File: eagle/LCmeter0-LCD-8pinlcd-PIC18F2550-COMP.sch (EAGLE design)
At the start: 35 parts, among them IC1 PIC18F2550-I/SP-COMP-B-V, J1 HD44780-4BITLCD44780-8P, J2 PIC-UART, J3 PIC-ICSP, J4 J4, J5 CONN-2P2P/V, J7 CONN-2P2P/V, K2 DS2Y, Q1 20MHz, SW1 PB-1P-1T, T1 BC547

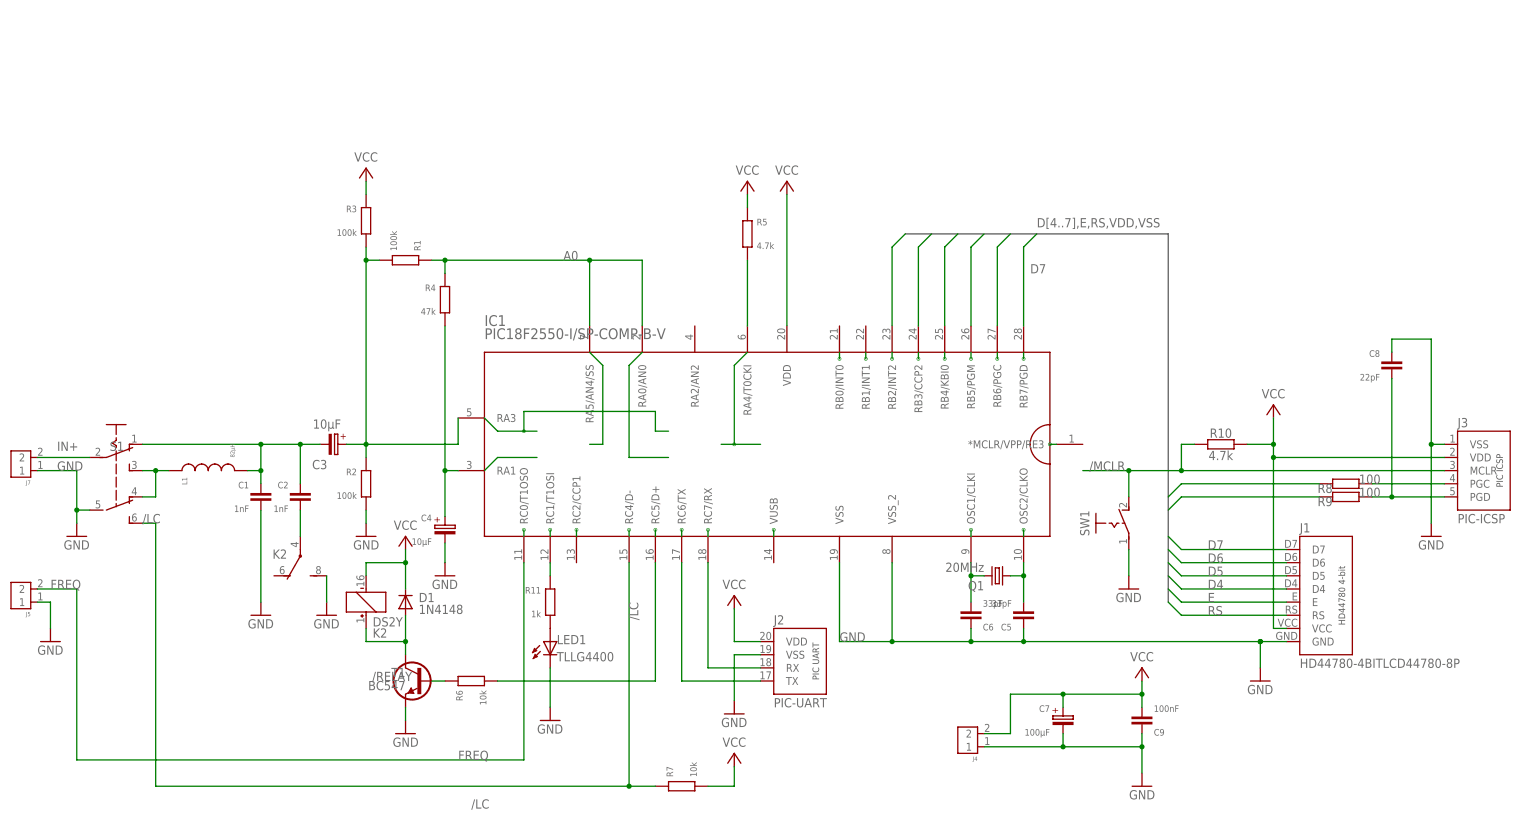
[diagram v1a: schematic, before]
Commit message: ...
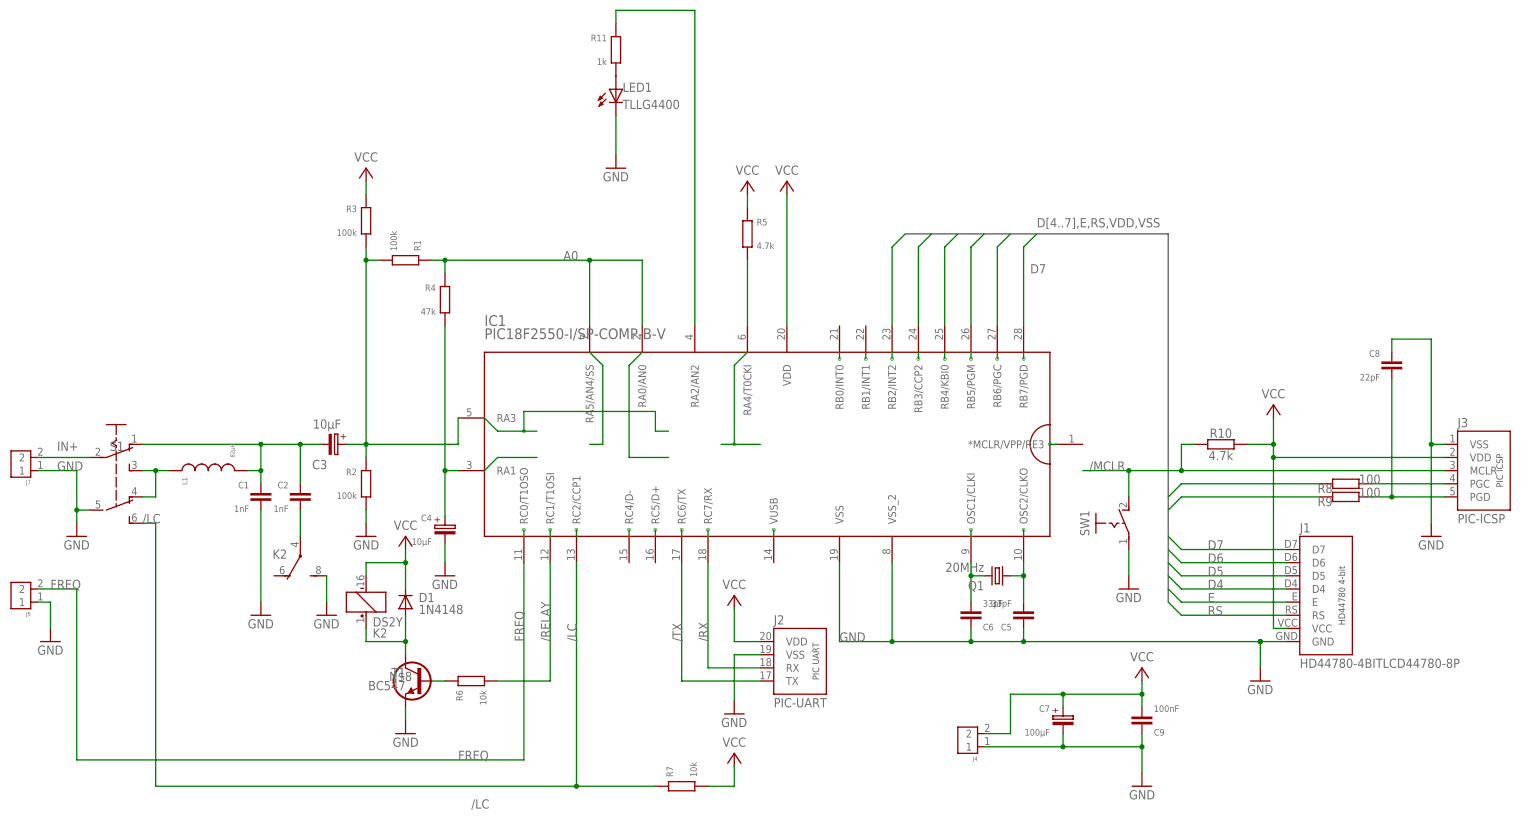
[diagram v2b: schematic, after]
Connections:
- net N$10 renamed /TX
- net N$9 renamed /RX
- net /LC: now also IC1.RC2/CCP1; no longer IC1.RC4/D-
- net /RELAY: now also IC1.RC1/T1OSI, R6.1; no longer D1.A, K21.+, T1.C
- net N$3: now also IC1.RA2/AN2; no longer IC1.RC1/T1OSI
- net N$8: now also D1.A, K21.+, T1.C; no longer IC1.RC5/D+, R6.1
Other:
- moved on the sheet: LED1, R11
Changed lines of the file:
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@@
 </instance>
 <instance part="J1" gate="G$1" x="228.6" y="0"/>
-<instance part="LED1" gate="G$1" x="86.36" y="-8.89" rot="MR0"/>
-<instance part="GND10" gate="1" x="86.36" y="-22.86"/>
+<instance part="LED1" gate="G$1" x="99.06" y="97.79" rot="MR0"/>
+<instance part="GND10" gate="1" x="99.06" y="83.82"/>
 <instance part="GND13" gate="1" x="200.66" y="-35.56" rot="MR0"/>
 <instance part="J4" gate="G$1" x="167.64" y="-27.94" rot="MR0"/>
@@
 </instance>
 <instance part="R6" gate="G$1" x="71.12" y="-15.24" rot="R90"/>
-<instance part="R11" gate="G$1" x="86.36" y="0"/>
+<instance part="R11" gate="G$1" x="99.06" y="106.68"/>
 <instance part="J7" gate="G$1" x="-15.24" y="25.4" rot="MR0"/>
 <instance part="J5" gate="G$1" x="-15.24" y="0" rot="MR0"/>
@@
 <pinref part="GND10" gate="1" pin="GND"/>
 <pinref part="LED1" gate="G$1" pin="C"/>
-<wire x1="86.36" y1="-12.7" x2="86.36" y2="-20.32" width="0.1524" layer="91"/>
+<wire x1="99.06" y1="93.98" x2="99.06" y2="86.36" width="0.1524" layer="91"/>
 </segment>
 <segment>
@@
 <pinref part="S1" gate="G$1" pin="S1"/>
 <wire x1="10.16" y1="15.24" x2="10.16" y2="-35.56" width="0.1524" layer="91"/>
-<wire x1="10.16" y1="-35.56" x2="101.6" y2="-35.56" width="0.1524" layer="91"/>
+<wire x1="10.16" y1="-35.56" x2="91.44" y2="-35.56" width="0.1524" layer="91"/>
 <label x="71.12" y="-38.1" size="1.778" layer="95" rot="MR180"/>
 <pinref part="R7" gate="G$1" pin="2"/>
-<wire x1="101.6" y1="7.62" x2="101.6" y2="-35.56" width="0.1524" layer="91"/>
-<wire x1="101.6" y1="-35.56" x2="106.68" y2="-35.56" width="0.1524" layer="91"/>
-<junction x="101.6" y="-35.56"/>
-<label x="101.6" y="0" size="1.778" layer="95" rot="R270"/>
-<pinref part="IC1" gate="G$1" pin="RC4/D-"/>
-</segment>
-</net>
-<net name="/RELAY" class="0">
+<pinref part="IC1" gate="G$1" pin="RC2/CCP1"/>
+<wire x1="91.44" y1="-35.56" x2="106.68" y2="-35.56" width="0.1524" layer="91"/>
+<wire x1="91.44" y1="-35.56" x2="91.44" y2="7.62" width="0.1524" layer="91"/>
+<junction x="91.44" y="-35.56"/>
+<label x="91.44" y="-7.62" size="1.778" layer="95" rot="R90"/>
+</segment>
+</net>
+<net name="N$8" class="0">
 <segment>
 <pinref part="T1" gate="G$1" pin="C"/>
@@
 <label x="68.58" y="-30.48" size="1.778" layer="95"/>
 <pinref part="IC1" gate="G$1" pin="RC0/T1OSO"/>
+<label x="81.28" y="-7.62" size="1.778" layer="95" rot="R90"/>
 </segment>
 </net>
@@
 </segment>
 </net>
-<net name="N$8" class="0">
+<net name="/RELAY" class="0">
 <segment>
 <pinref part="R6" gate="G$1" pin="1"/>
-<wire x1="76.2" y1="-15.24" x2="106.68" y2="-15.24" width="0.1524" layer="91"/>
-<wire x1="106.68" y1="-15.24" x2="106.68" y2="7.62" width="0.1524" layer="91"/>
-<pinref part="IC1" gate="G$1" pin="RC5/D+"/>
-</segment>
-</net>
-<net name="N$9" class="0">
+<wire x1="76.2" y1="-15.24" x2="86.36" y2="-15.24" width="0.1524" layer="91"/>
+<pinref part="IC1" gate="G$1" pin="RC1/T1OSI"/>
+<wire x1="86.36" y1="7.62" x2="86.36" y2="-15.24" width="0.1524" layer="91"/>
+<label x="86.36" y="-7.62" size="1.778" layer="95" rot="R90"/>
+</segment>
+</net>
+<net name="/RX" class="0">
 <segment>
 <pinref part="J2" gate="1" pin="RX"/>
@@
 <wire x1="116.84" y1="-12.7" x2="116.84" y2="7.62" width="0.1524" layer="91"/>
 <pinref part="IC1" gate="G$1" pin="RC7/RX"/>
-</segment>
-</net>
-<net name="N$10" class="0">
+<label x="116.84" y="-7.62" size="1.778" layer="95" rot="R90"/>
+</segment>
+</net>
+<net name="/TX" class="0">
 <segment>
 <pinref part="J2" gate="1" pin="TX"/>
@@
 <wire x1="111.76" y1="-15.24" x2="127" y2="-15.24" width="0.1524" layer="91"/>
 <pinref part="IC1" gate="G$1" pin="RC6/TX"/>
+<label x="111.76" y="-7.62" size="1.778" layer="95" rot="R90"/>
 </segment>
 </net>
@@
 <net name="N$3" class="0">
 <segment>
+<pinref part="IC1" gate="G$1" pin="RA2/AN2"/>
+<wire x1="114.3" y1="53.34" x2="114.3" y2="114.3" width="0.1524" layer="91"/>
 <pinref part="R11" gate="G$1" pin="2"/>
-<pinref part="IC1" gate="G$1" pin="RC1/T1OSI"/>
-<wire x1="86.36" y1="5.08" x2="86.36" y2="7.62" width="0.1524" layer="91"/>
-</segment>
-</net>
+<wire x1="114.3" y1="114.3" x2="99.06" y2="114.3" width="0.1524" layer="91"/>
+<wire x1="99.06" y1="114.3" x2="99.06" y2="111.76" width="0.1524" layer="91"/>
+</segment>
+</net>
